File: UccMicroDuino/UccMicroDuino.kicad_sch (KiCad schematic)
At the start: 8 parts, among them J2 Conn_01x10_Socket, J2 USB_A, U2 ATtiny85-20S

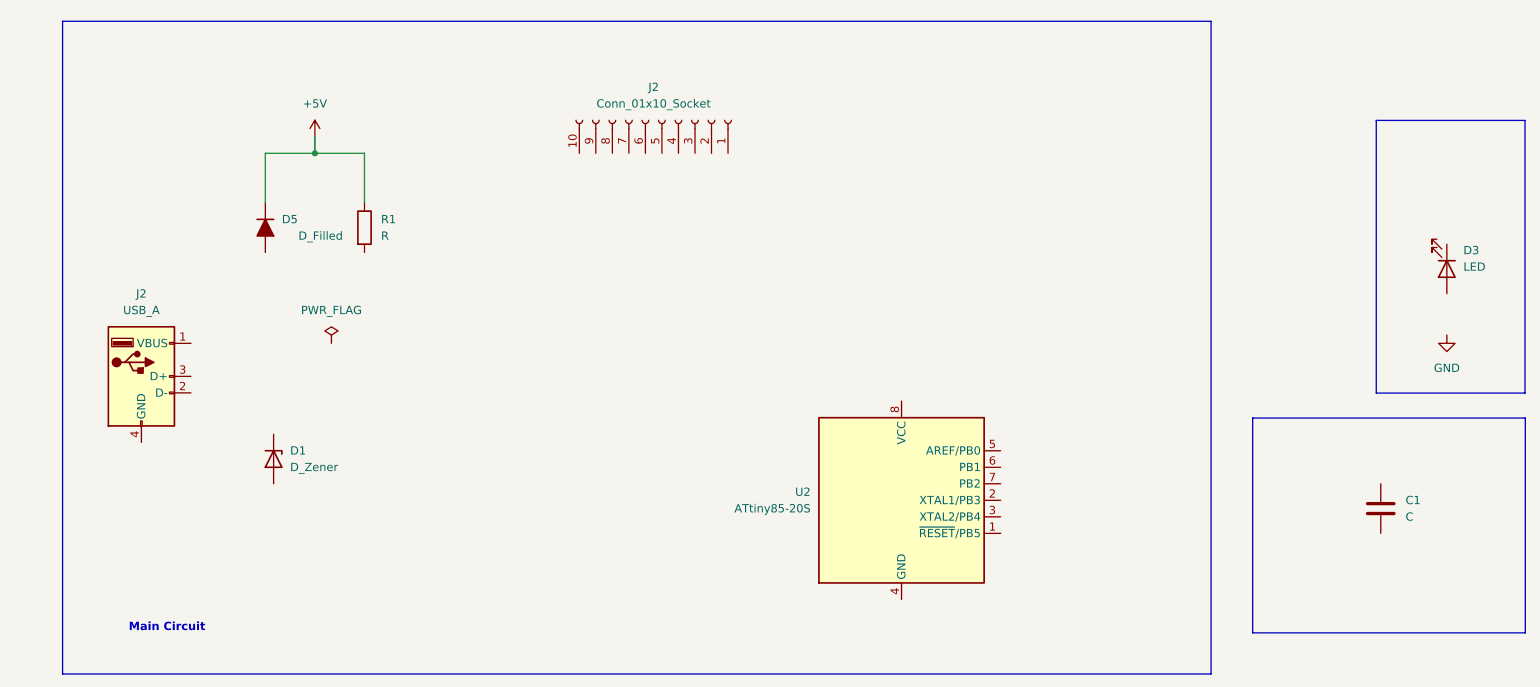
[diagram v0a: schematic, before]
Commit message: first class
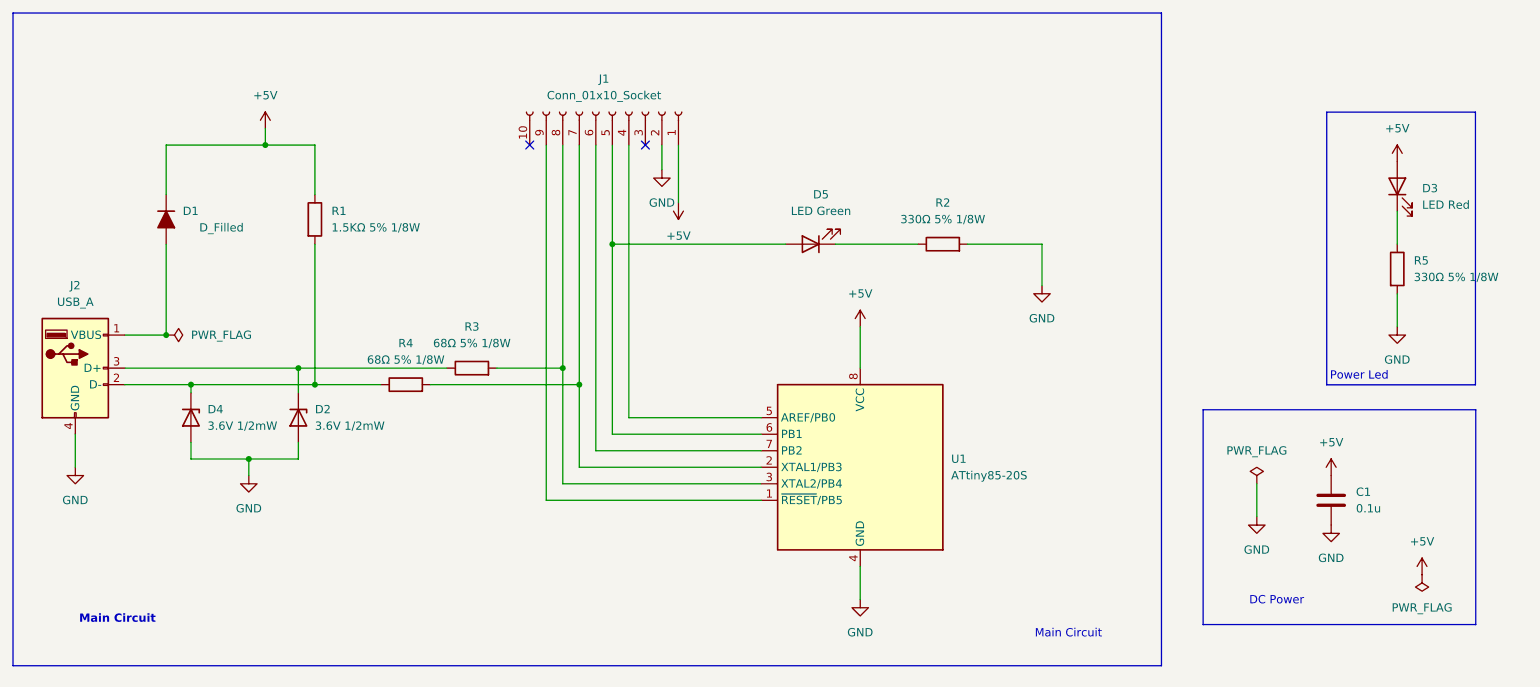
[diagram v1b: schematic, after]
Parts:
- added D4: 3.6V 1/2mW, symbol Device:D_Zener
- added D5: LED Green, symbol Device:LED
- added R2, R5: 330Ω 5% 1/8W, symbol Device:R
- added R3, R4: 68Ω 5% 1/8W, symbol Device:R
- C1: value C -> 0.1u
- D2: renamed from D1; value D_Zener -> 3.6V 1/2mW
- D3: value LED -> LED Red
- R1: value R -> 1.5KΩ 5% 1/8W
- renumbered D5 to D1, J2 to J1, U2 to U1
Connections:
- net +5V: now also C1.1, D3.2 (A), J1.1 (Pin_1), U1.8 (VCC)
- net GND: now also C1.2, D2.2 (A), J1.2 (Pin_2), J2.4 (GND), U1.4 (GND), D4.2 (A), R2.2, R5.2
- net at D3.1 (K): now also R5.1
- net at R1.2: now also J2.2 (D-), D4.1 (K), R4.1
- net at D2.1 (K): now also J2.3 (D+), R3.1
- net at U1.1 (~{RESET}/PB5): now also J1.9 (Pin_9)
- net at U1.2 (XTAL1/PB3): now also J1.7 (Pin_7), R4.2
- net at U1.3 (XTAL2/PB4): now also J1.8 (Pin_8), R3.2
- net at U1.5 (AREF/PB0): now also J1.4 (Pin_4)
- net at U1.6 (PB1): now also J1.5 (Pin_5), D5.2 (A)
- net at U1.7 (PB2): now also J1.6 (Pin_6)
- net at J2.1 (VBUS): now also D1.2 (A)
- new net: D5.1 (K), R2.1
- no-connect marks 0 -> 2
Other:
- note added: "DC Power"
- note added: "Power Led"
- moved on the sheet: C1, D1, D2, D3, J1, J2, R1, U1
